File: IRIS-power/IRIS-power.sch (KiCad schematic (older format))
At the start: 7 parts, among them J11 Powerpole

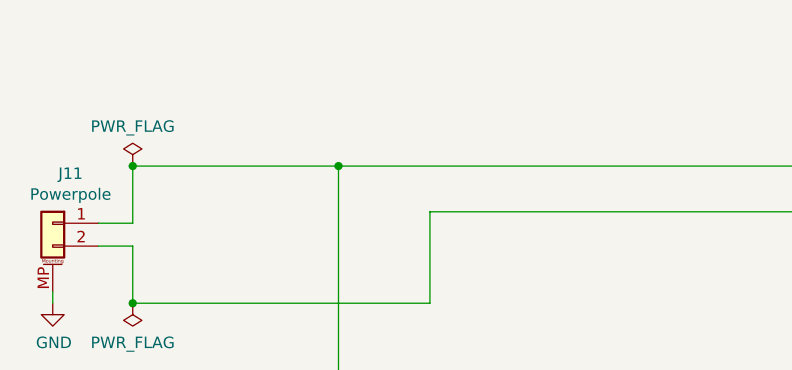
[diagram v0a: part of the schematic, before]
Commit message: IRIS V4.02
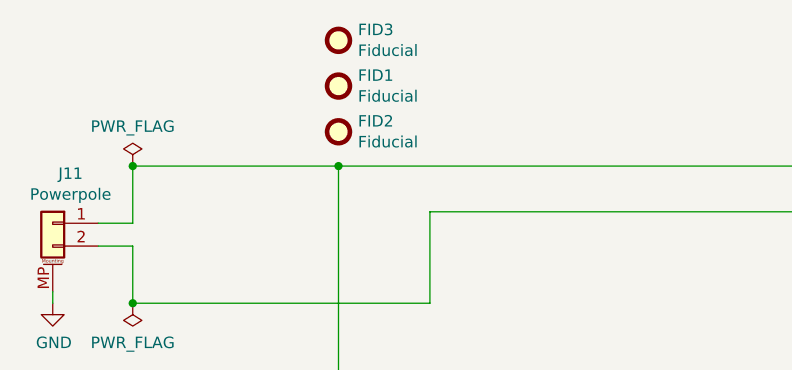
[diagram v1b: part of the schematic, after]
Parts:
- added FID1, FID2, FID3: Fiducial, Fiducial:Fiducial_1.5mm_Mask3mm, symbol Mechanical:Fiducial
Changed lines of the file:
@@
 Wire Wire Line
 	2000 5550 2600 5550
+$Comp
+L Mechanical:Fiducial FID2
+U 1 1 5FD5D545
+P 2200 2150
+F 0 "FID2" H 2285 2196 50  0000 L CNN
+F 1 "Fiducial" H 2285 2105 50  0000 L CNN
+F 2 "Fiducial:Fiducial_1.5mm_Mask3mm" H 2200 2150 50  0001 C CNN
+F 3 "~" H 2200 2150 50  0001 C CNN
+	1    2200 2150
+	1    0    0    -1
+$EndComp
+$Comp
+L Mechanical:Fiducial FID1
+U 1 1 5FD5DDFA
+P 2200 1950
+F 0 "FID1" H 2285 1996 50  0000 L CNN
+F 1 "Fiducial" H 2285 1905 50  0000 L CNN
+F 2 "Fiducial:Fiducial_1.5mm_Mask3mm" H 2200 1950 50  0001 C CNN
+F 3 "~" H 2200 1950 50  0001 C CNN
+	1    2200 1950
+	1    0    0    -1
+$EndComp
+$Comp
+L Mechanical:Fiducial FID3
+U 1 1 5FD618C3
+P 2200 1750
+F 0 "FID3" H 2285 1796 50  0000 L CNN
+F 1 "Fiducial" H 2285 1705 50  0000 L CNN
+F 2 "Fiducial:Fiducial_1.5mm_Mask3mm" H 2200 1750 50  0001 C CNN
+F 3 "~" H 2200 1750 50  0001 C CNN
+	1    2200 1750
+	1    0    0    -1
+$EndComp
 $EndSCHEMATC
